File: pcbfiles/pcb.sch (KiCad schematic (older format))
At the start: 236 parts, among them J1 Conn_01x04_Female, J10 Conn_01x05, J2 Conn_01x05, J3 Conn_01x05, J4 Conn_01x05, J5 Conn_01x05, J6 Conn_01x04_Female, J7 Conn_01x05, J8 Conn_01x05, J9 Conn_01x05, Q1 AO3401A, Q2 AO3401A, SW1 SW_SPST, SW10 SW_SPST, SW11 SW_SPST, SW12 SW_SPST, SW13 SW_SPST, SW14 SW_SPST, SW15 SW_SPST, SW16 SW_SPST, SW17 SW_SPST, SW18 SW_SPST, SW19 SW_SPST, SW2 SW_SPST, SW20 SW_SPST, SW21 SW_SPST, SW22 SW_SPST, SW23 SW_SPST, SW24 SW_SPST, SW25 SW_SPST, SW26 SW_SPST, SW27 SW_SPST, SW28 SW_SPST, SW29 SW_SPST, SW3 SW_SPST, SW30 SW_SPST, SW31 SW_SPST, SW32 SW_SPST, SW33 SW_SPST, SW34 SW_SPST, SW35 SW_SPST, SW36 SW_SPST, SW37 SW_SPST, SW38 SW_SPDT, SW39 SW_SPST, SW4 SW_SPST, SW40 SW_SPST, SW41 SW_SPST, SW42 SW_SPST, SW43 SW_SPST, SW44 SW_SPST, SW45 SW_SPST, SW46 Rotary_Encoder_Switch, SW47 SW_SPDT, SW48 SW_SPST, SW49 SW_SPST, SW5 SW_SPST, SW50 SW_SPST, SW51 SW_SPST, SW52 SW_SPST, SW53 SW_SPST, SW54 SW_SPST, SW55 SW_SPST, SW56 SW_SPST, SW57 SW_SPST, SW58 SW_SPST, SW59 SW_SPST, SW6 SW_SPST, SW60 SW_SPST, SW61 SW_SPST, SW62 SW_SPST, SW63 SW_SPST, SW64 SW_SPST, SW65 SW_SPST, SW66 SW_SPST, SW67 SW_SPST, SW68 SW_SPST, SW69 SW_SPST, SW7 SW_SPST, SW70 SW_SPST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

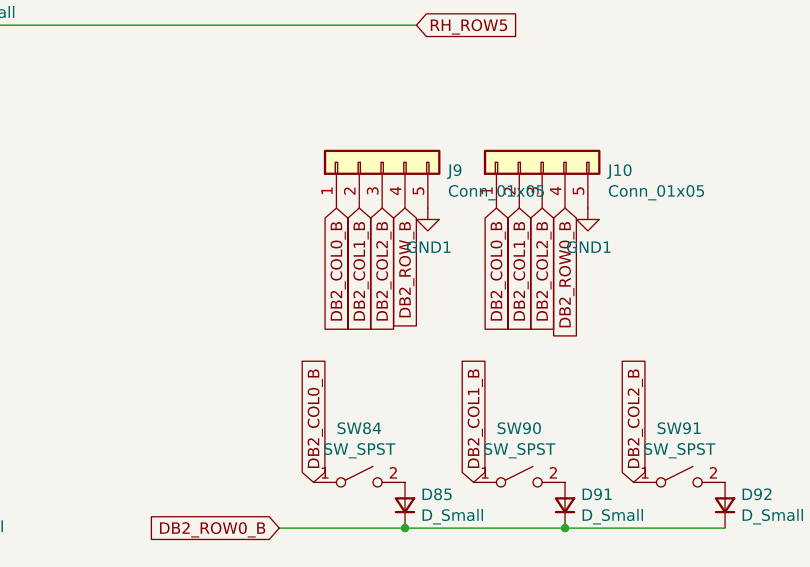
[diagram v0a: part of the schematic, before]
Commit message: Final commit for the day.
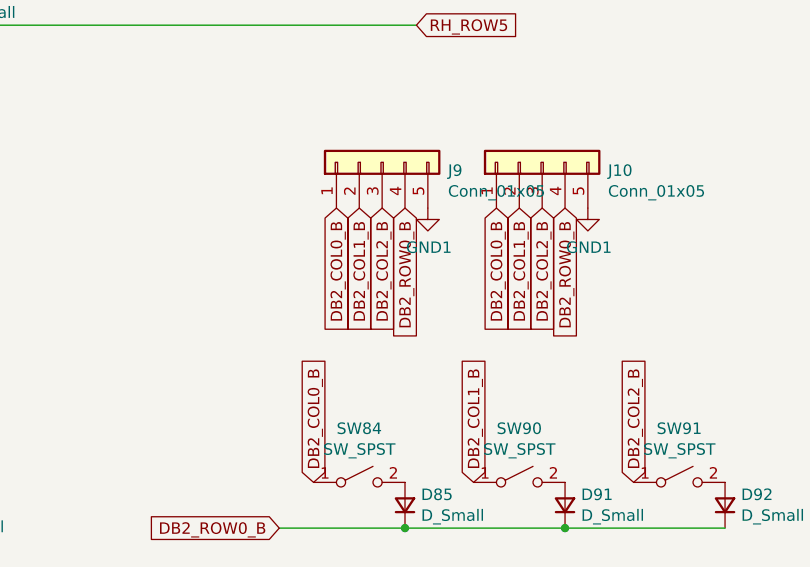
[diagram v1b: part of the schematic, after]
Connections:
- net DB2_ROW_B is gone; now on net DB2_ROW0_B: J9.4 (Pin_4)
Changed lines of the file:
@@
 DB2_COL2_B
 Text GLabel 25750 6700 3    50   Input ~ 0
-DB2_ROW_B
+DB2_ROW0_B
 $Comp
 L power:GND1 #PWR0133
